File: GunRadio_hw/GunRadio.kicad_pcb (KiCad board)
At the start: 2 copper layers, 24.4 x 77.7 mm, 41 parts

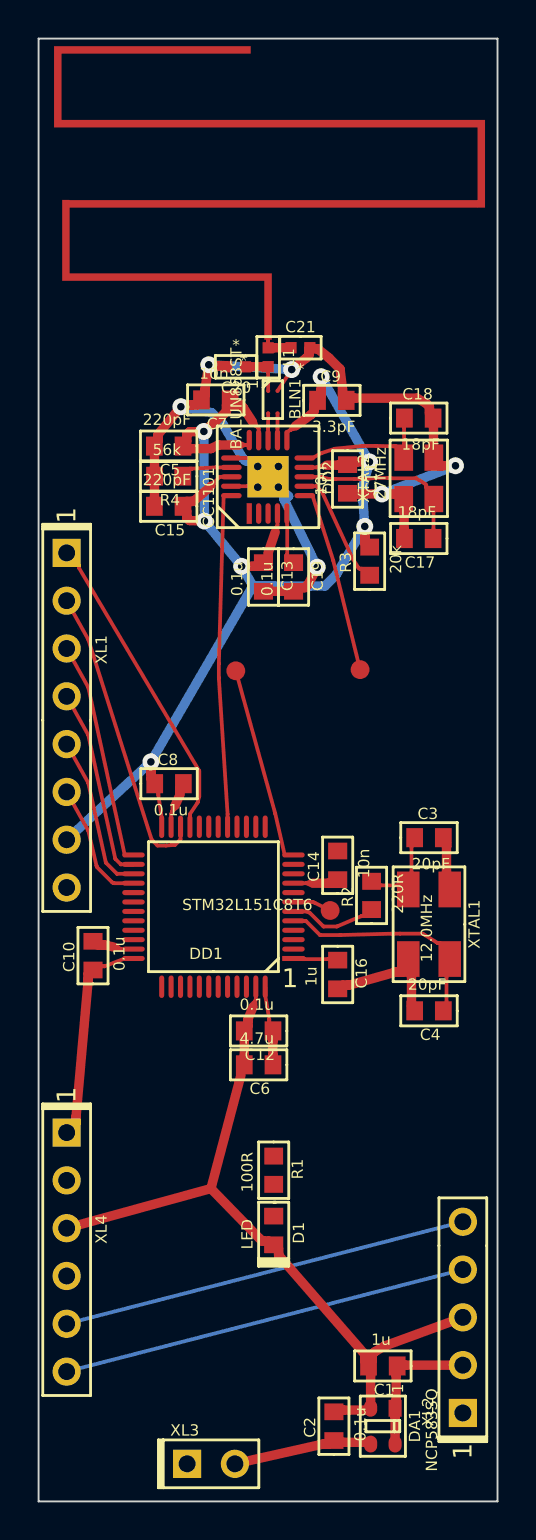
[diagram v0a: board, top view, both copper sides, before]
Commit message: GunRadio finished
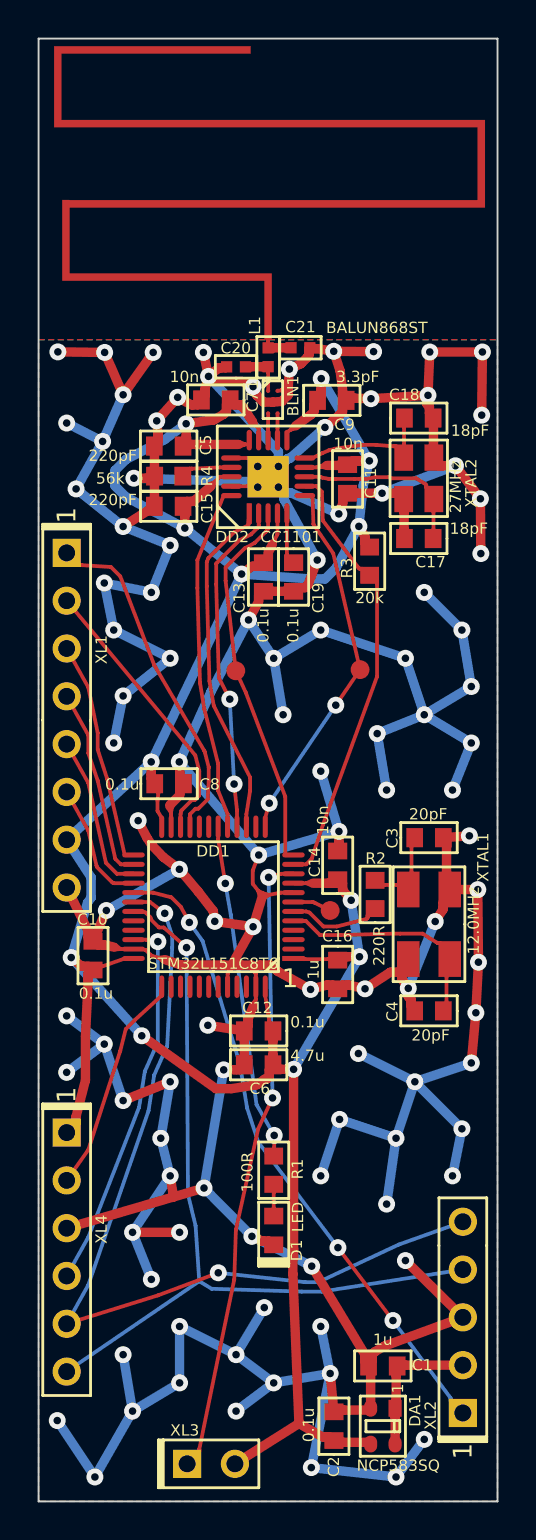
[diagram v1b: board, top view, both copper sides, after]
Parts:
- moved R2 0.20 mm to (145.4, 125.5)
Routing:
- net GND: track 115.4 -> 427.8 mm, vias 6 -> 106
- net +3.3V: track 106.6 -> 167.1 mm, vias 7 -> 12
- net /Trigger: track 0.00 -> 34.1 mm, vias 0 -> 3
- net Net-(DD1-Pad10): track 0.00 -> 33.3 mm, vias 0 -> 2
- net /UART_TX: track 21.7 -> 46.9 mm, vias 0 -> 2
- net /UART_RX: track 21.7 -> 44.1 mm, vias 0 -> 1
- net /SWDIO: track 0.00 -> 20.0 mm, vias 0 -> 1
- net /CC_SCK: track 0.00 -> 18.2 mm
- net Net-(DD1-Pad18): track 0.00 -> 17.9 mm, vias 0 -> 2
- net /CC_MISO: track 0.00 -> 17.9 mm, vias 0 -> 2
- net /CC_CS: track 6.26 -> 23.4 mm
- net /SWCLK: track 0.00 -> 11.8 mm
- net /CC_GDO0: track 10.00 -> 20.0 mm, vias 0 -> 2
- net /CC_GDO2: track 10.6 -> 20.1 mm
- net Net-(D1-PadA): track 0.00 -> 1.69 mm
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- added copper zone on B.Cu, net GND
- added copper zone on F.Cu, net GND
